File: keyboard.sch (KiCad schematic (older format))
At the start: 12 parts, among them J1 CONN_01X05, J2 USB_A, J3 CONN_02X03, U1 ATMEGA32U4-AU, Y1 16mhz

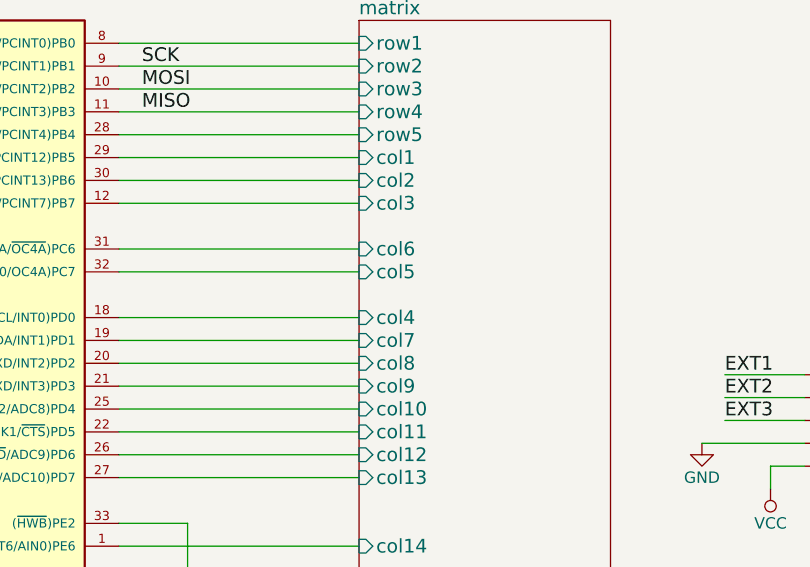
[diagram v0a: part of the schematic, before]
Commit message: checkpoint
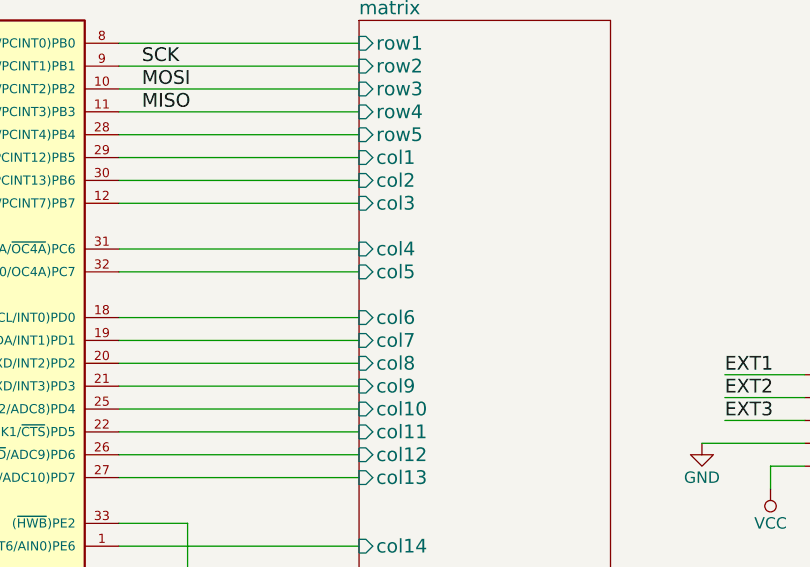
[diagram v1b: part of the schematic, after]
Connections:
- net matrix/col4: now also U1.31 ((OC3A/~OC4A~)PC6); no longer U1.18 ((OC0B/SCL/INT0)PD0)
- net matrix/col6: now also U1.18 ((OC0B/SCL/INT0)PD0); no longer U1.31 ((OC3A/~OC4A~)PC6)
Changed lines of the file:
@@
 F8 "col2" I L 9450 2100 60
 F9 "col3" I L 9450 2200 60
-F10 "col4" I L 9450 2700 60
+F10 "col4" I L 9450 2400 60
 F11 "col5" I L 9450 2500 60
-F12 "col6" I L 9450 2400 60
+F12 "col6" I L 9450 2700 60
 F13 "col7" I L 9450 2800 60
 F14 "col8" I L 9450 2900 60

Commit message: new net list
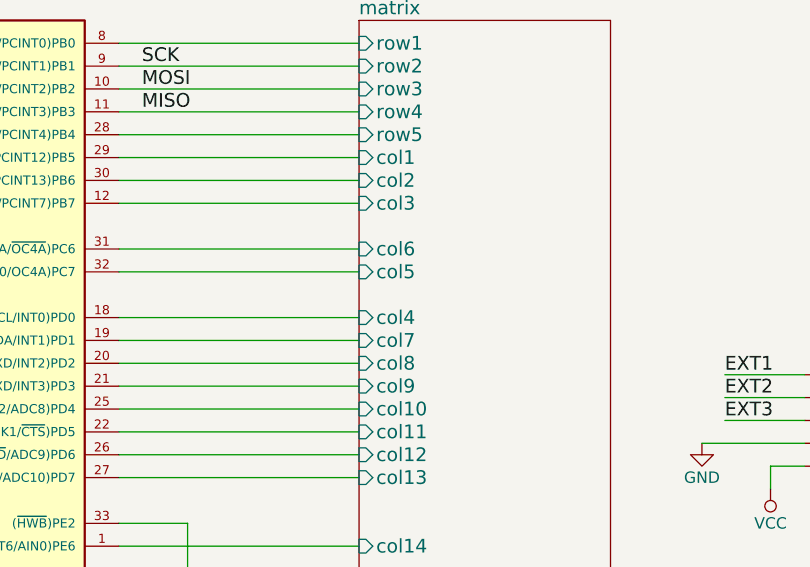
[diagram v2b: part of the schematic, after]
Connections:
- net matrix/col4: now also U1.18 ((OC0B/SCL/INT0)PD0); no longer U1.31 ((OC3A/~OC4A~)PC6)
- net matrix/col6: now also U1.31 ((OC3A/~OC4A~)PC6); no longer U1.18 ((OC0B/SCL/INT0)PD0)
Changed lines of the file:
@@
 F8 "col2" I L 9450 2100 60
 F9 "col3" I L 9450 2200 60
-F10 "col4" I L 9450 2400 60
+F10 "col4" I L 9450 2700 60
 F11 "col5" I L 9450 2500 60
-F12 "col6" I L 9450 2700 60
+F12 "col6" I L 9450 2400 60
 F13 "col7" I L 9450 2800 60
 F14 "col8" I L 9450 2900 60
